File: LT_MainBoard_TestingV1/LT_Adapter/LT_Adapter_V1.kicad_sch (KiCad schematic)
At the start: 10 parts, among them CN1 NUCLEO-L432KC, U1 317990687

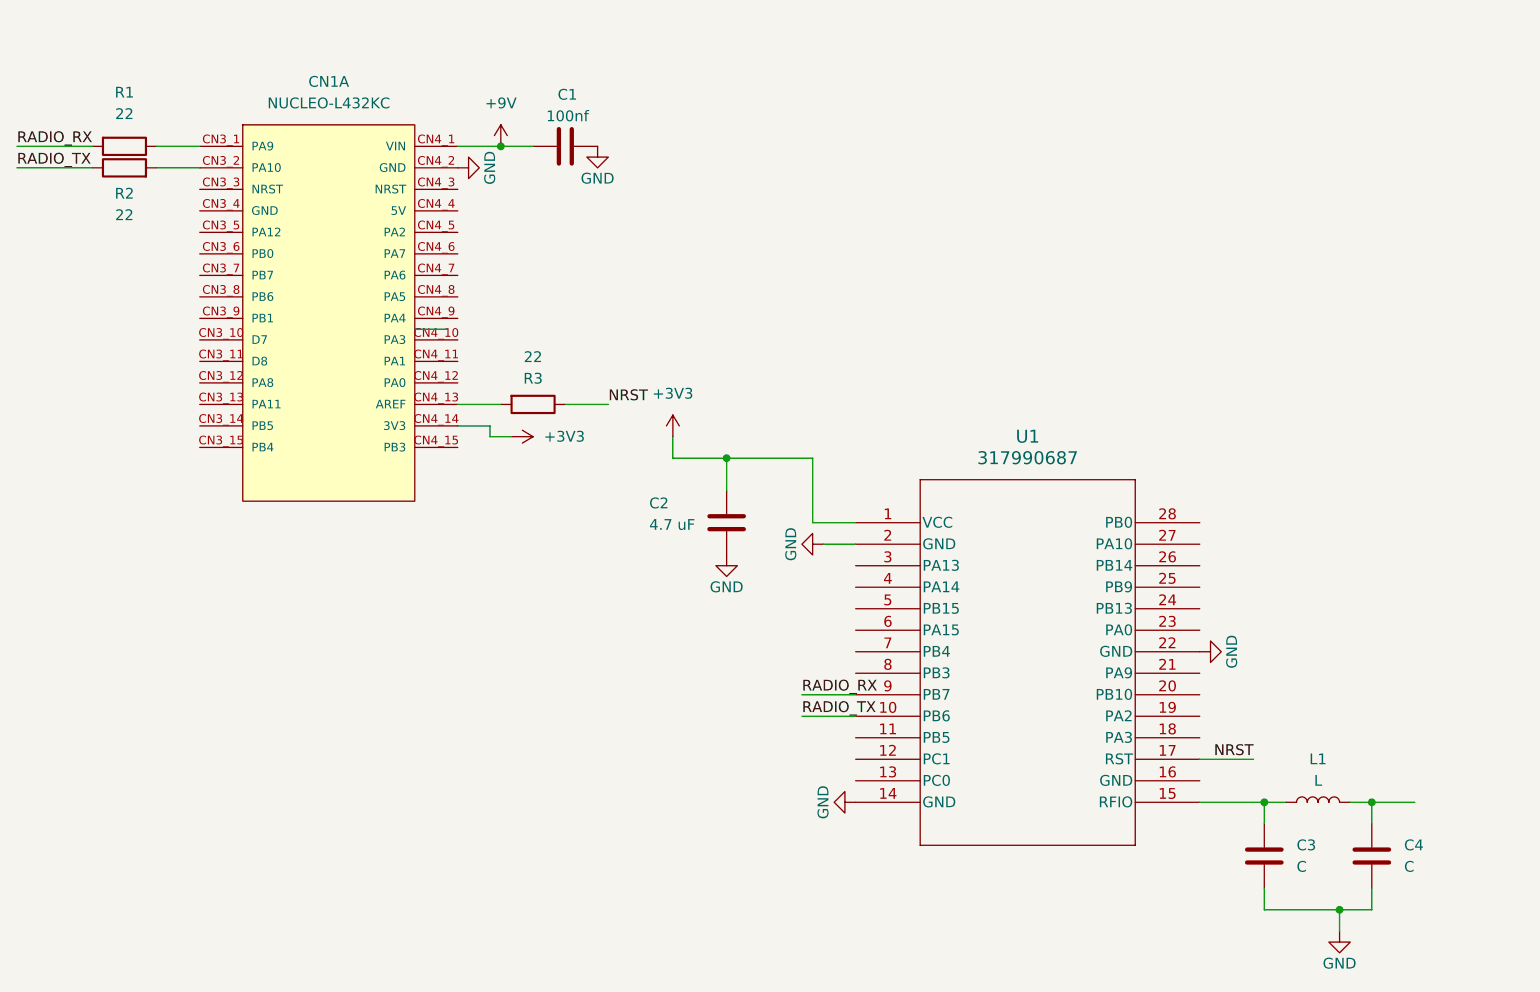
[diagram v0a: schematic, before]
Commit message: Adaptor PCB
Version 1
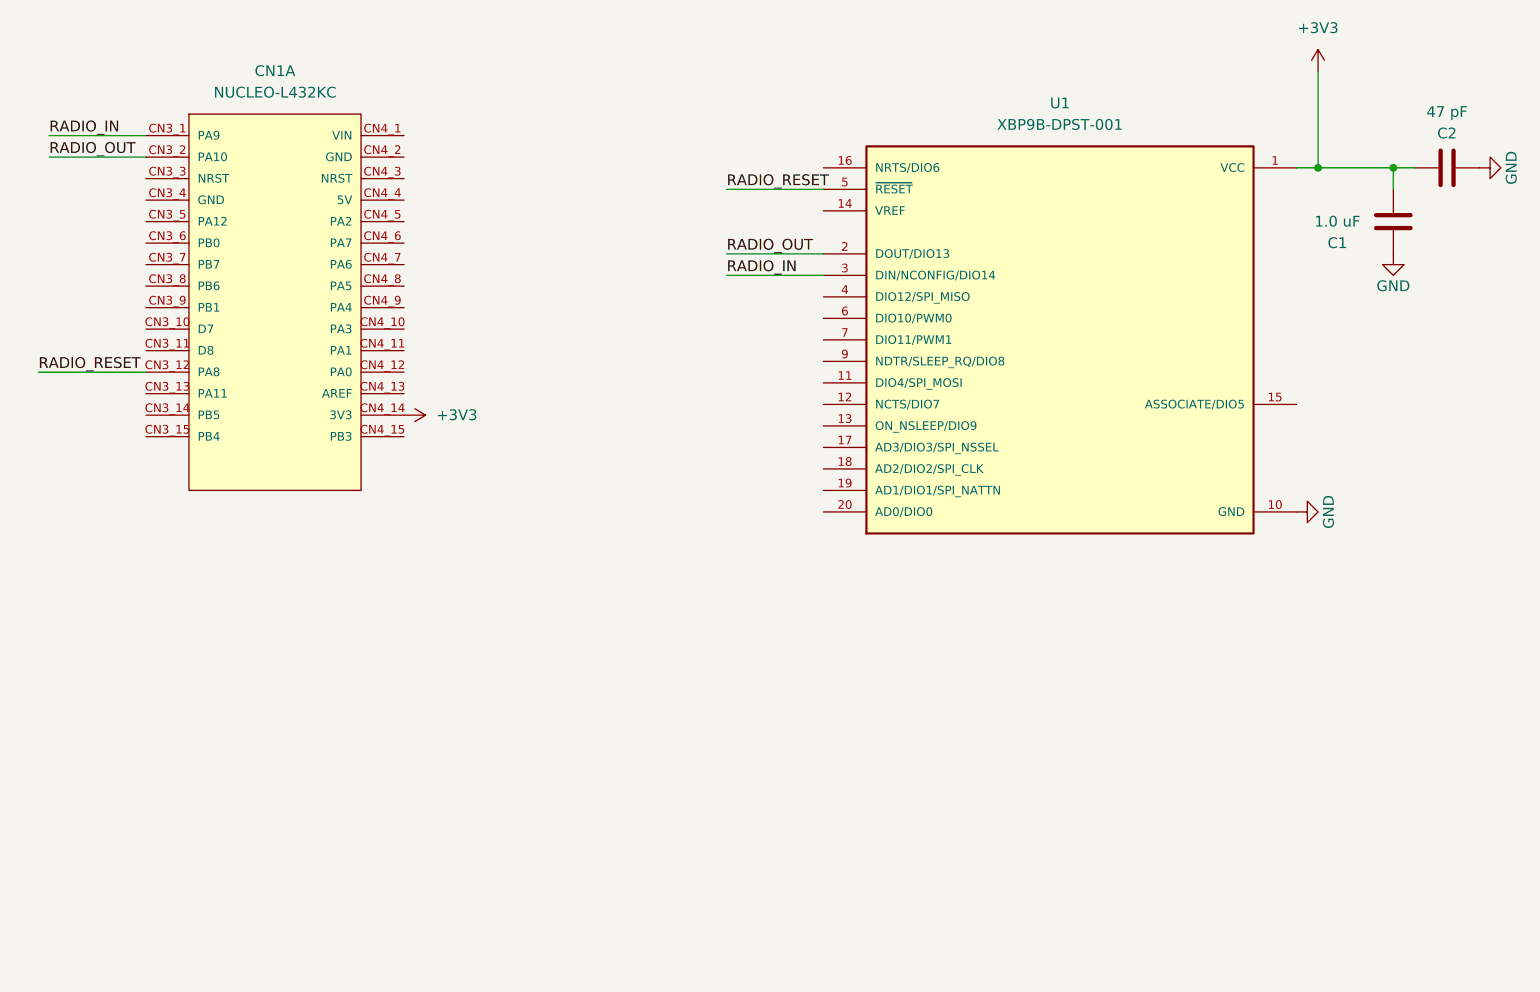
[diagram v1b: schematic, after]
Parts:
- removed C3, C4: C, symbol Device:C
- removed L1: L, symbol Device:L
- removed R1, R2, R3: 22, symbol Device:R
- removed U1: 317990687, QFN_90687_SEE, symbol FS_3_Global_Symbol_Library:SEEED317990687
- added U1: XBP9B-DPST-001, XBP9B-DPST-001:DIP2200W51P200L3294H279Q20P, symbol FS_3_Global_Symbol_Library:XBP9B-DPST-001
- C1: value 100nf -> 1.0 uF
- C2: value 4.7 uF -> 47 pF; footprint (none) -> Capacitor_SMD:C_0805_2012Metric_Pad1.18x1.45mm_HandSolder
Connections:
- net +3V3: now also C1.1, U1.1 (VCC)
- net GND: now also U1.10 (GND); no longer CN1.CN4_2 (GND)
- net RADIO_IN: now reaches CN1.CN3_1 (PA9)
- net RADIO_IN: now also U1.3 (DIN/NCONFIG/DIO14)
- net RADIO_RESET: now reaches CN1.CN3_12 (PA8)
- net RADIO_RESET: now also U1.5 (~{RESET})
- net RADIO_OUT: now reaches CN1.CN3_2 (PA10)
- net RADIO_OUT: now also U1.2 (DOUT/DIO13)
- net +9V: no longer names the net of CN1.CN4_1 (VIN)
- net +9V: no longer C1.1
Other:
- moved on the sheet: CN1A
